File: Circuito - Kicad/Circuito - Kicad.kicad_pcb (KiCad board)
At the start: 2 copper layers, 5 parts, among them U1 4N25

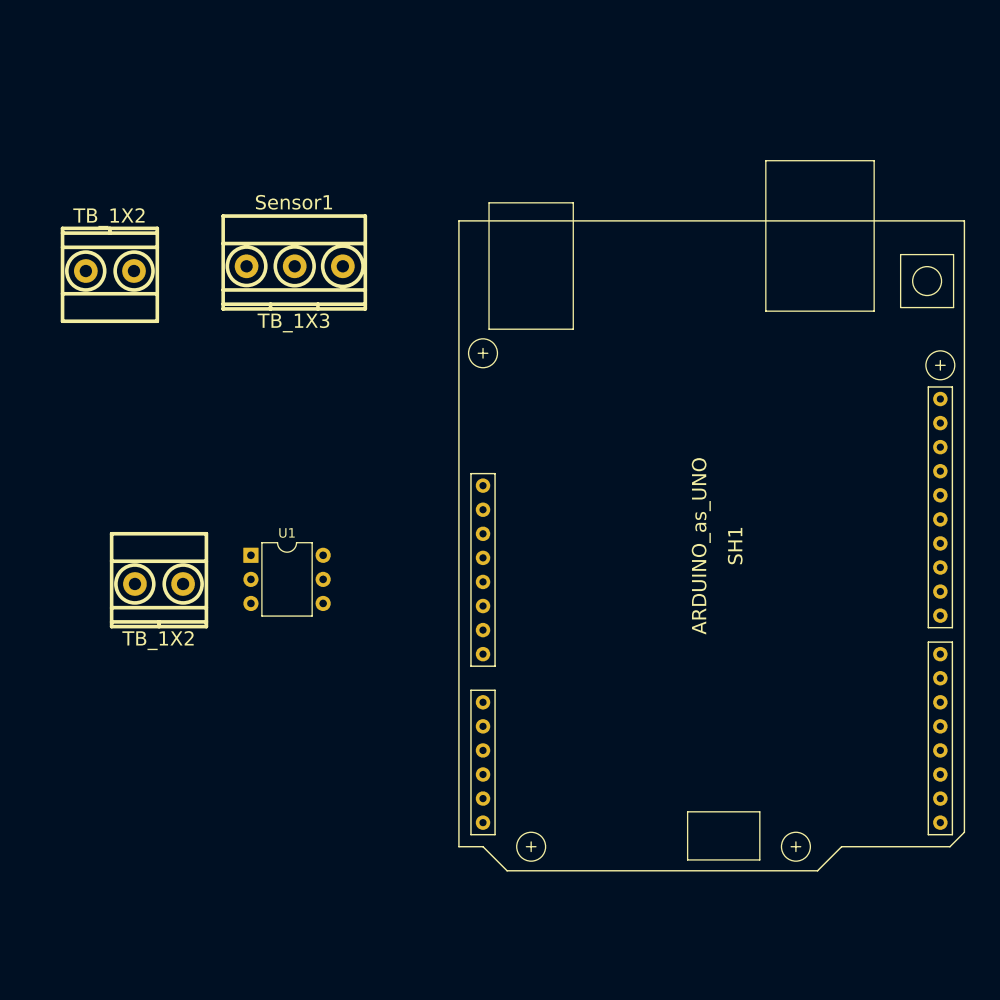
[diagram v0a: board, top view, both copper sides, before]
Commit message: Kicad | PCB Improvement
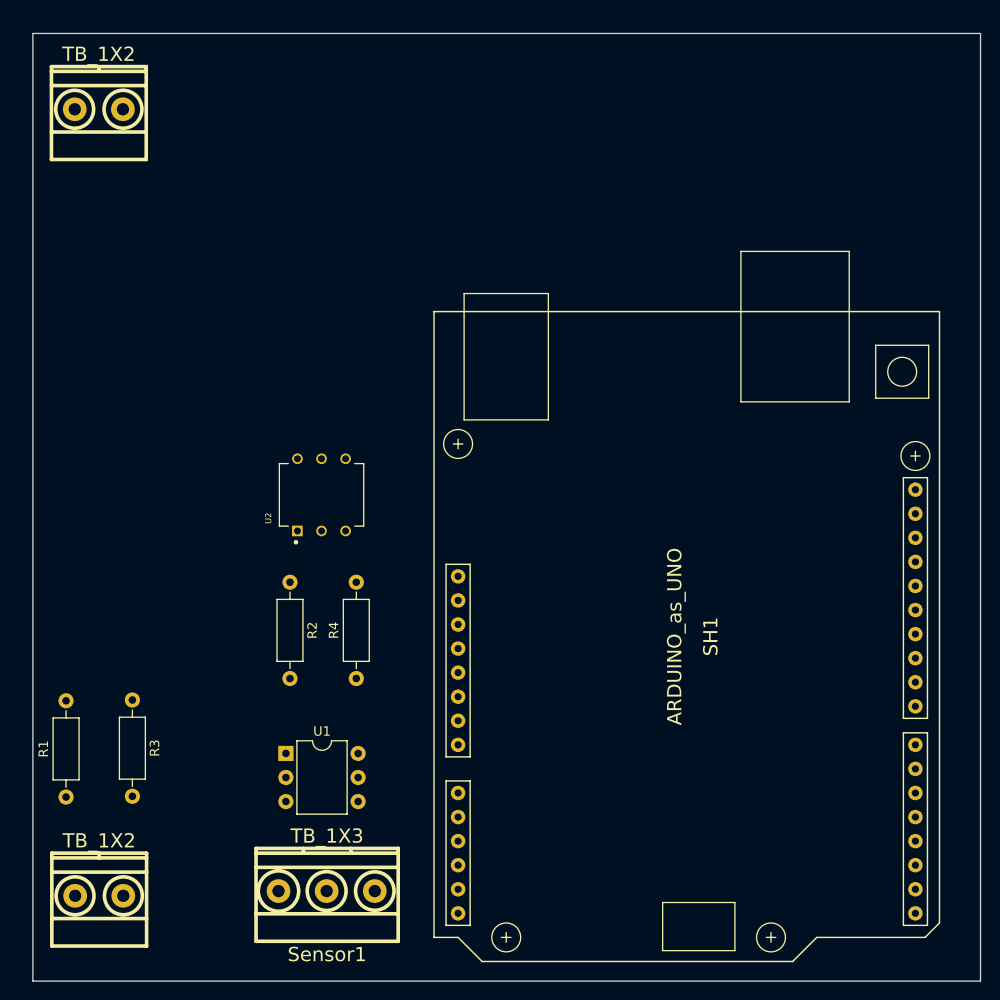
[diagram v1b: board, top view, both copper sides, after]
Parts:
- added R1: 100, Resistor_THT:R_Axial_DIN0207_L6.3mm_D2.5mm_P10.16mm_Horizontal, F.Cu at (104.4, 130.0)
- added R2: 100, Resistor_THT:R_Axial_DIN0207_L6.3mm_D2.5mm_P10.16mm_Horizontal, F.Cu at (128.0, 107.3)
- added R3: 100k, Resistor_THT:R_Axial_DIN0207_L6.3mm_D2.5mm_P10.16mm_Horizontal, F.Cu at (111.4, 119.8)
- added R4: 10k, Resistor_THT:R_Axial_DIN0207_L6.3mm_D2.5mm_P10.16mm_Horizontal, F.Cu at (135.0, 117.5)
- added U2: MOC3021M, MOC3021:DIP762W45P254L889H508Q6, F.Cu at (131.3, 98.1)
- moved Sensor1 66.0 mm to (131.9, 139.9), turned to 180 degrees
- moved Calentador1 33.5 mm to (107.9, 140.4), turned to 180 degrees
- moved U1 21.2 mm to (127.6, 125.4)
- moved Alterna1 17.1 mm to (107.8, 57.4)
- moved SH1 9.92 mm to (169.9, 113.1)
- renumbered AC1 to Alterna1
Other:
- board outline added: 100 x 100 mm

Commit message: Kicad | PCB Added
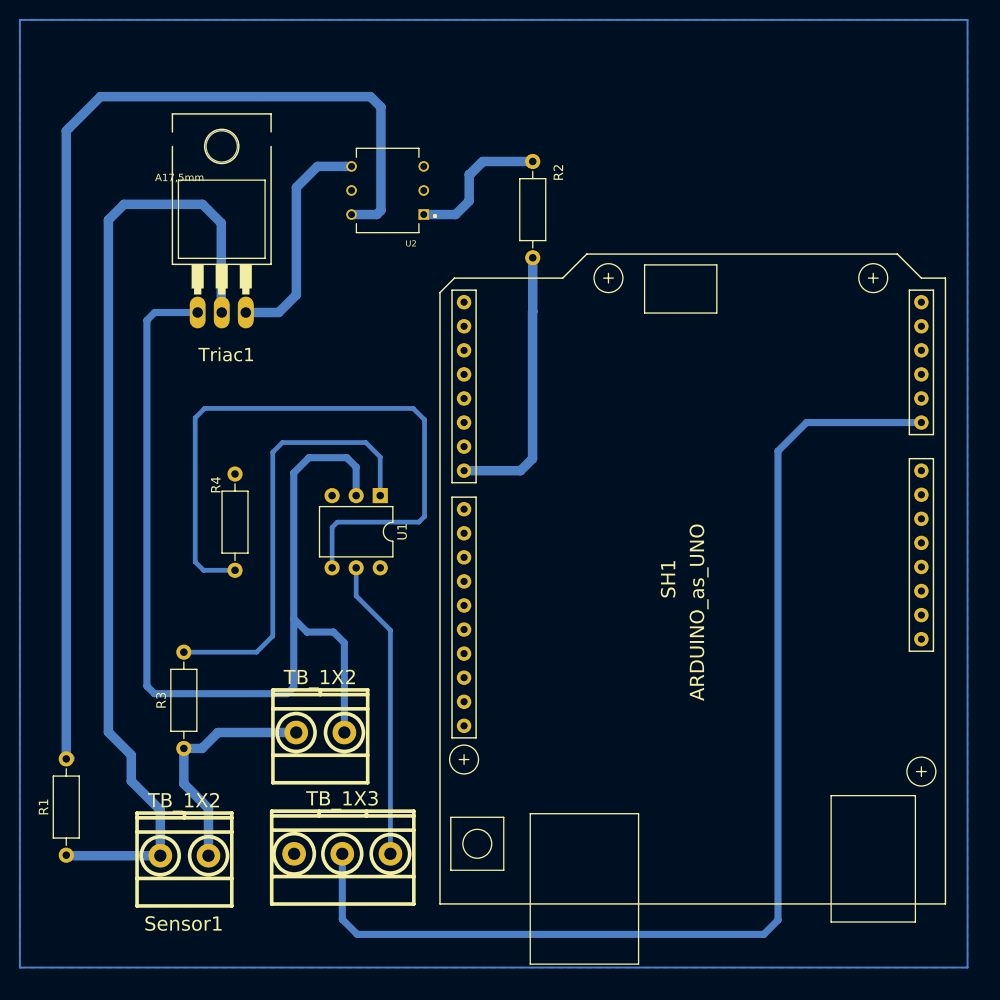
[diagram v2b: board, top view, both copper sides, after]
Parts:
- added Triac1: Generic_Triac_A1A2G, BT136:TO220AB, F.Cu at (120.8, 72.5)
- moved Alterna1 69.8 mm to (131.2, 123.2)
- moved R2 51.3 mm to (153.6, 62.9)
- moved U2 32.9 mm to (138.3, 66.0), turned to 180 degrees
- moved U1 29.0 mm to (137.5, 98.2), turned to -90 degrees
- moved R4 17.2 mm to (122.2, 106.1)
- moved Calentador1 9.94 mm to (116.9, 136.2)
- moved R3 7.46 mm to (116.8, 124.9), turned to 90 degrees
- moved R1 6.13 mm to (104.4, 136.1)
- moved SH1 6.10 mm to (170.5, 107.0), turned to 90 degrees
- moved Sensor1 4.26 mm to (133.5, 136.0)
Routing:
- net PIN_A0: track 0.00 -> 120.1 mm
- net Net-(R1-Pad2): track 0.00 -> 115.8 mm
- net Vivo: track 0.00 -> 109.5 mm
- net Net-(Triac1-A2): track 0.00 -> 102.2 mm
- net Net-(R4-Pad1): track 0.00 -> 69.6 mm
- net Net-(R3-Pad2): track 0.00 -> 46.0 mm
- net VCC: track 0.00 -> 31.7 mm
- net PIN_7: track 0.00 -> 29.0 mm
- net Neutro: track 0.00 -> 25.0 mm
- net Net-(Triac1-G): track 0.00 -> 24.2 mm
- net Net-(R2-Pad1): track 0.00 -> 17.2 mm
- added copper zone on B.Cu, net GND
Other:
- board outline removed
